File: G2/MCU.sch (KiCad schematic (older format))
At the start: 23 parts, among them CON401 AVR-JTAG-10, J401 Conn_01x07, J402 Conn_02x08_Odd_Even, J403 Conn_02x04_Counter_Clockwise, U401 TXB0102DCU

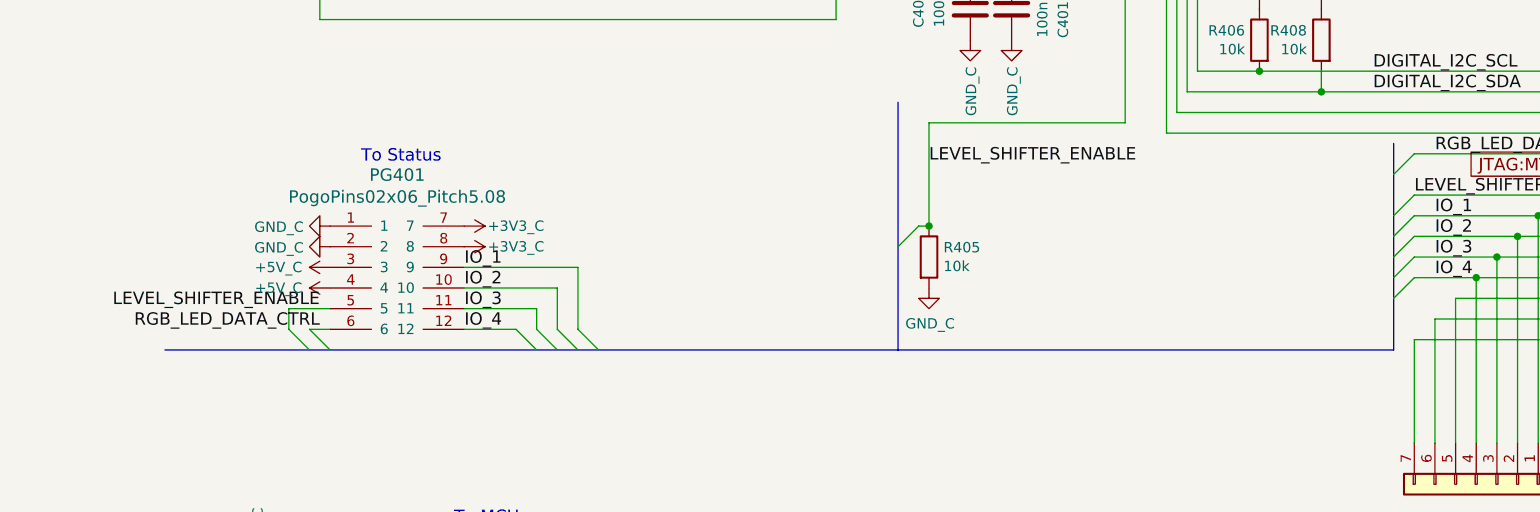
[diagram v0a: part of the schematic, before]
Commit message: No longer uses Pogo pins
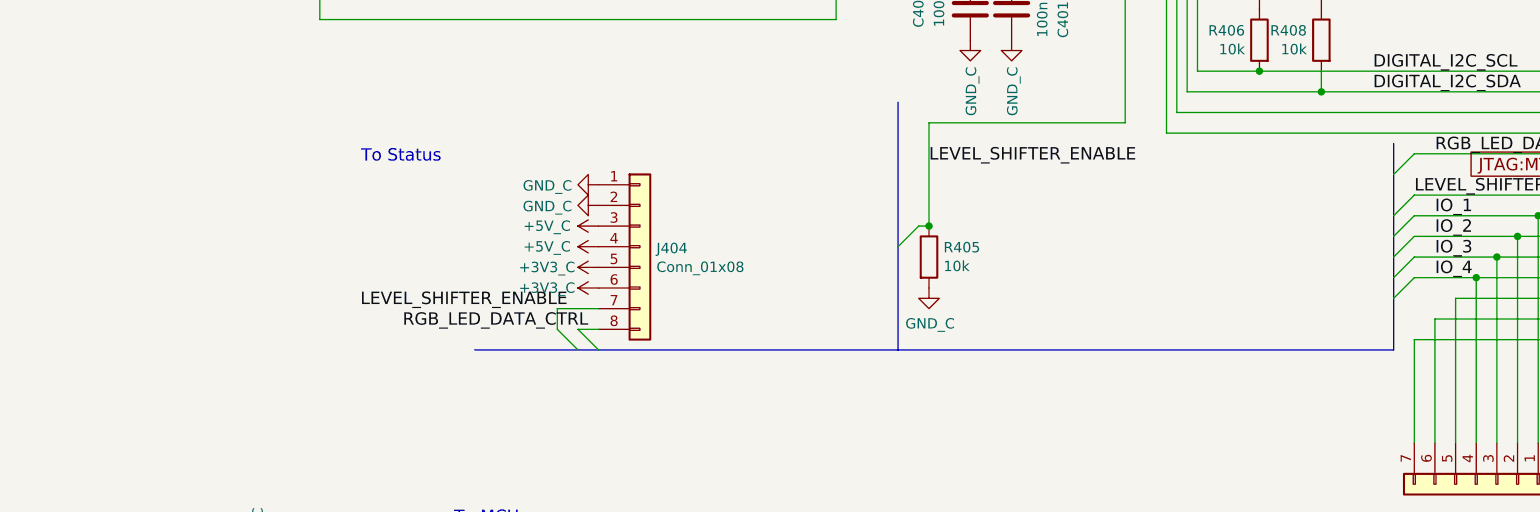
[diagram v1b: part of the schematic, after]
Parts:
- removed PG401: PogoPins02x06_Pitch5.08, PogoPins02x06_Pitch5:PogoPins02x06_Pitch5.08, symbol PogoPins02x06_Pitch5.08
- added J404: Conn_01x08, LocalComponents:WE68710814022_8x0.50mm_SMT_ZIF_Horizontal_Top, symbol Conn_01x08
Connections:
- net +3V3_C: now also J404.5 (Pin_5), J404.6 (Pin_6)
- net +5V_C: now also J404.3 (Pin_3), J404.4 (Pin_4)
- net GND_C: now also J404.1 (Pin_1), J404.2 (Pin_2)
- net LEVEL_SHIFTER_ENABLE: now also J404.7 (Pin_7)
- net RGB_LED_DATA_CTRL: now also J404.8 (Pin_8)
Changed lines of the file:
@@
 Text Label 3550 2750 2    60   ~ 0
 DIGITAL_I2C_SCL
-Text Label 2650 5050 2    60   ~ 0
+Text Label 3850 5050 2    60   ~ 0
 LEVEL_SHIFTER_ENABLE
-Text Label 2650 5150 2    60   ~ 0
+Text Label 3950 5150 2    60   ~ 0
 RGB_LED_DATA_CTRL
 Entry Wire Line
-	2600 5150 2700 5250
-Entry Wire Line
-	2500 5150 2600 5250
+	3900 5150 4000 5250
+Entry Wire Line
+	3800 5150 3900 5250
 Entry Wire Line
 	7850 4400 7950 4300
@@
 L GND_C #PWR075
 U 1 1 59CA6266
-P 2700 4650
-F 0 "#PWR075" H 2700 4400 50  0001 C CNN
-F 1 "GND_C" V 2705 4522 50  0000 R CNN
-F 2 "" H 2700 4650 50  0001 C CNN
-F 3 "" H 2700 4650 50  0001 C CNN
-	1    2700 4650
+P 4000 4450
+F 0 "#PWR075" H 4000 4200 50  0001 C CNN
+F 1 "GND_C" V 4005 4322 50  0000 R CNN
+F 2 "" H 4000 4450 50  0001 C CNN
+F 3 "" H 4000 4450 50  0001 C CNN
+	1    4000 4450
 	0    1    1    0
 $EndComp
@@
 L GND_C #PWR076
 U 1 1 59CA62B6
-P 2700 4750
-F 0 "#PWR076" H 2700 4500 50  0001 C CNN
-F 1 "GND_C" V 2705 4622 50  0000 R CNN
-F 2 "" H 2700 4750 50  0001 C CNN
-F 3 "" H 2700 4750 50  0001 C CNN
-	1    2700 4750
+P 4000 4550
+F 0 "#PWR076" H 4000 4300 50  0001 C CNN
+F 1 "GND_C" V 4005 4422 50  0000 R CNN
+F 2 "" H 4000 4550 50  0001 C CNN
+F 3 "" H 4000 4550 50  0001 C CNN
+	1    4000 4550
 	0    1    1    0
 $EndComp
@@
 L +3V3_C #PWR0122
 U 1 1 59CA73CD
-P 3350 4750
-F 0 "#PWR0122" H 3350 4600 50  0001 C CNN
-F 1 "+3V3_C" V 3350 5000 50  0000 C CNN
-F 2 "" H 3350 4750 50  0001 C CNN
-F 3 "" H 3350 4750 50  0001 C CNN
-	1    3350 4750
-	0    1    -1   0
+P 4000 4850
+F 0 "#PWR0122" H 4000 4700 50  0001 C CNN
+F 1 "+3V3_C" V 4000 5100 50  0000 C CNN
+F 2 "" H 4000 4850 50  0001 C CNN
+F 3 "" H 4000 4850 50  0001 C CNN
+	1    4000 4850
+	0    -1   1    0
 $EndComp
 $Comp
 L +3V3_C #PWR0123
 U 1 1 59CA7406
-P 3350 4650
-F 0 "#PWR0123" H 3350 4500 50  0001 C CNN
-F 1 "+3V3_C" V 3350 4900 50  0000 C CNN
-F 2 "" H 3350 4650 50  0001 C CNN
-F 3 "" H 3350 4650 50  0001 C CNN
-	1    3350 4650
-	0    1    -1   0
+P 4000 4950
+F 0 "#PWR0123" H 4000 4800 50  0001 C CNN
+F 1 "+3V3_C" V 4000 5200 50  0000 C CNN
+F 2 "" H 4000 4950 50  0001 C CNN
+F 3 "" H 4000 4950 50  0001 C CNN
+	1    4000 4950
+	0    -1   1    0
 $EndComp
 $Comp
 L +5V_C #PWR0124
 U 1 1 59CA75DF
-P 2700 4850
-F 0 "#PWR0124" H 2700 4700 50  0001 C CNN
-F 1 "+5V_C" V 2700 5100 50  0000 C CNN
-F 2 "" H 2700 4850 50  0001 C CNN
-F 3 "" H 2700 4850 50  0001 C CNN
-	1    2700 4850
+P 4000 4650
+F 0 "#PWR0124" H 4000 4500 50  0001 C CNN
+F 1 "+5V_C" V 4000 4900 50  0000 C CNN
+F 2 "" H 4000 4650 50  0001 C CNN
+F 3 "" H 4000 4650 50  0001 C CNN
+	1    4000 4650
 	0    -1   -1   0
 $EndComp
@@
 L +5V_C #PWR0125
 U 1 1 59CA770A
-P 2700 4950
-F 0 "#PWR0125" H 2700 4800 50  0001 C CNN
-F 1 "+5V_C" V 2700 5200 50  0000 C CNN
-F 2 "" H 2700 4950 50  0001 C CNN
-F 3 "" H 2700 4950 50  0001 C CNN
-	1    2700 4950
+P 4000 4750
+F 0 "#PWR0125" H 4000 4600 50  0001 C CNN
+F 1 "+5V_C" V 4000 5000 50  0000 C CNN
+F 2 "" H 4000 4750 50  0001 C CNN
+F 3 "" H 4000 4750 50  0001 C CNN
+	1    4000 4750
 	0    -1   -1   0
 $EndComp
@@
 Text Notes 3300 6100 0    60   ~ 0
 To MCU
-$Comp
-L PogoPins02x06_Pitch5.08 PG401
-U 1 1 59CF7820
-P 2900 4550
-F 0 "PG401" H 3025 4697 60  0000 C CNN
-F 1 "PogoPins02x06_Pitch5.08" H 3025 4591 60  0000 C CNN
-F 2 "PogoPins02x06_Pitch5:PogoPins02x06_Pitch5.08" H 2900 4550 60  0001 C CNN
-F 3 "" H 2900 4550 60  0001 C CNN
-	1    2900 4550
-	1    0    0    -1
-$EndComp
 $Comp
 L Conn_01x07 J401
@@
 Text Label 8600 5200 0    60   ~ 0
 IO_7
-Entry Wire Line
-	3900 5150 4000 5250
-Entry Wire Line
-	3800 5150 3900 5250
-Entry Wire Line
-	3700 5150 3800 5250
-Entry Wire Line
-	3600 5150 3700 5250
-Text Label 3350 4850 0    60   ~ 0
-IO_1
-Text Label 3350 4950 0    60   ~ 0
-IO_2
-Text Label 3350 5050 0    60   ~ 0
-IO_3
-Text Label 3350 5150 0    60   ~ 0
-IO_4
 Text Label 5600 4350 0    60   ~ 0
 LEVEL_SHIFTER_ENABLE
@@
 	8950 4350 8950 4400
 Wire Wire Line
-	2600 5150 2700 5150
-Wire Wire Line
-	2500 5150 2500 5050
-Wire Wire Line
-	2500 5050 2700 5050
+	3900 5150 4000 5150
+Wire Wire Line
+	3800 5150 3800 5050
+Wire Wire Line
+	3800 5050 4000 5050
 Wire Wire Line
 	5600 4650 5550 4650
@@
 Wire Wire Line
 	4900 3150 4900 2150
-Wire Bus Line
-	1900 5250 7850 5250
 Wire Wire Line
 	7950 4600 8950 4600
@@
 Connection ~ 8250 4900
 Wire Wire Line
-	3600 5150 3350 5150
-Wire Wire Line
-	3350 5050 3700 5050
-Wire Wire Line
-	3350 4950 3800 4950
-Wire Wire Line
-	3350 4850 3900 4850
-Wire Wire Line
-	3700 5050 3700 5150
-Wire Wire Line
-	3800 4950 3800 5150
-Wire Wire Line
-	3900 4850 3900 5150
-Wire Wire Line
 	5350 1450 5350 1500
 Wire Wire Line
@@
 Wire Wire Line
 	6800 2850 6300 2850
+$Comp
+L Conn_01x08 J404
+U 1 1 5A081331
+P 4200 4750
+F 0 "J404" H 4280 4742 50  0000 L CNN
+F 1 "Conn_01x08" H 4280 4651 50  0000 L CNN
+F 2 "LocalComponents:WE68710814022_8x0.50mm_SMT_ZIF_Horizontal_Top" H 4200 4750 50  0001 C CNN
+F 3 "https://www.mouser.se/Search/ProductDetail.aspx?qs=ZtY9WdtwX54hJHBraEAPJw%3d%3d" H 4200 4750 50  0001 C CNN
+	1    4200 4750
+	1    0    0    -1
+$EndComp
+Wire Bus Line
+	3400 5250 7850 5250
 $EndSCHEMATC
